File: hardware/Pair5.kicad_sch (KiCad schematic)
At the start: 10 parts, among them IC5 TPS2HCS08AQPWPRQ1, J16 Conn_01x02, J8 Conn_01x02

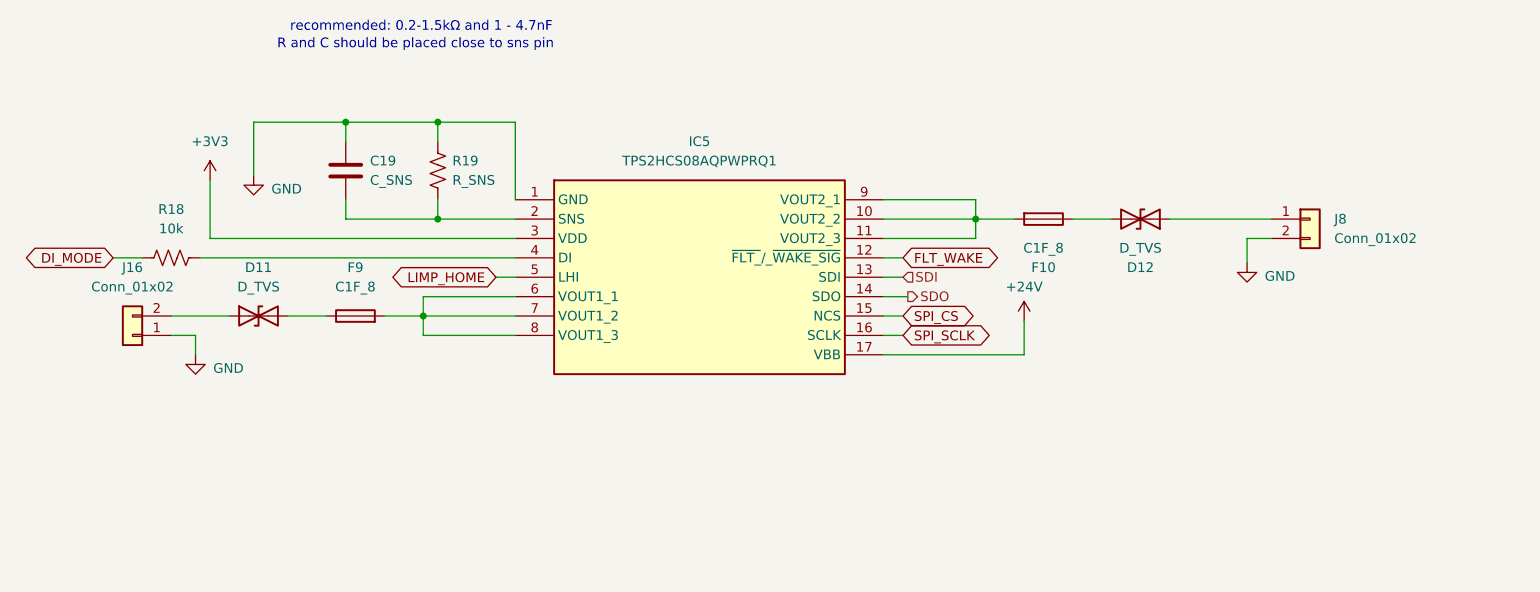
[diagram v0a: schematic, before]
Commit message: aesthetic added
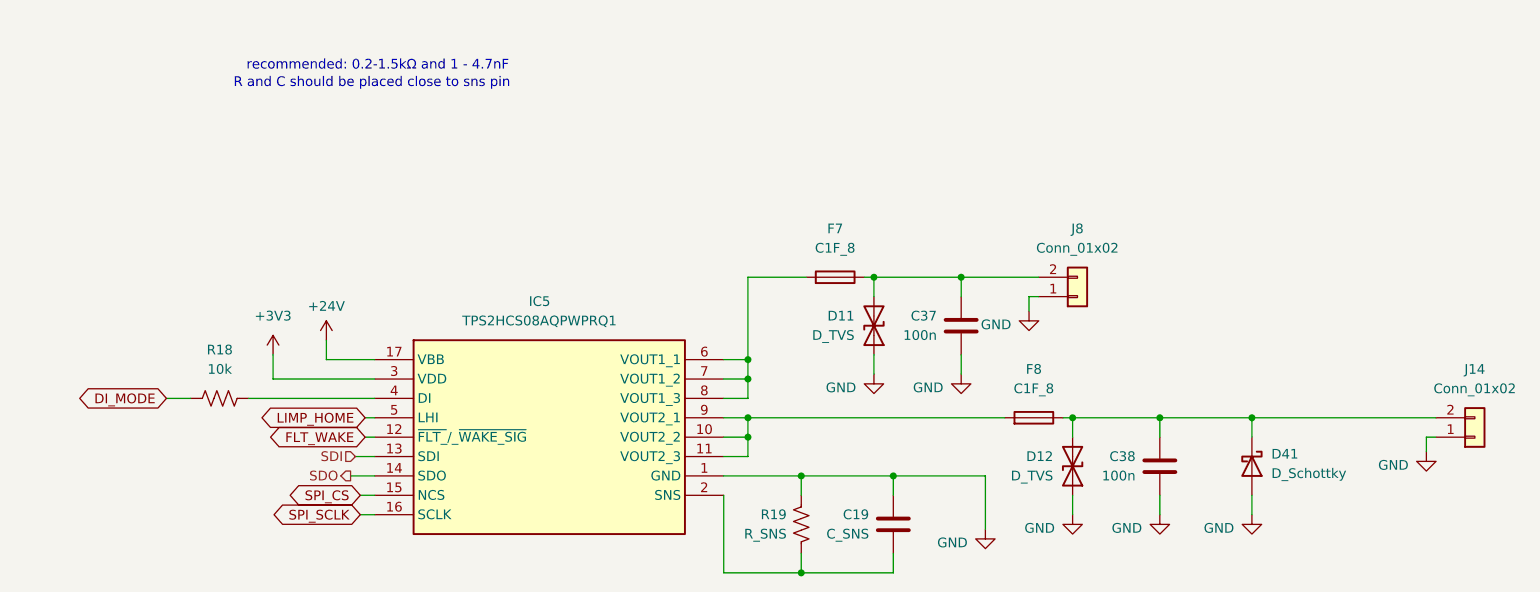
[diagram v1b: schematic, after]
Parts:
- removed F10, F9: C1F_8, Fuse:Fuse_1206_3216Metric, symbol PowerDistributionUnitLib:C1F_8
- removed J16: Conn_01x02, symbol Connector_Generic:Conn_01x02
- added C37, C38: 100n, symbol Device:C
- added D41: D_Schottky, symbol Device:D_Schottky
- added F7, F8: C1F_8, Fuse:Fuse_1206_3216Metric, symbol PowerDistributionUnitLib:C1F_8
- added J14: Conn_01x02, symbol Connector_Generic:Conn_01x02
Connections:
- net GND: now also D11.1 (A1), D12.1 (A1), J8.1 (Pin_1), C37.1, C38.1, D41.2 (A), J14.1 (Pin_1); no longer J8.2 (Pin_2)
- net at D12.2 (A2): now also C38.2, D41.1 (K), F8.1, J14.2 (Pin_2)
- net at IC5.10 (VOUT2_2), IC5.11 (VOUT2_3), IC5.9 (VOUT2_1): now also F8.2
- net at IC5.6 (VOUT1_1), IC5.7 (VOUT1_2), IC5.8 (VOUT1_3): now also F7.2
- net at D11.2 (A2): now also J8.2 (Pin_2), C37.2, F7.1
